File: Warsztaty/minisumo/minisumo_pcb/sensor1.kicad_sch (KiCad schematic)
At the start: 7 parts, among them U5 VL53L0CXV0DH1

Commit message: chyba gotowy schemat
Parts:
- C21, C22: footprint (none) -> Capacitor_SMD:C_0805_2012Metric_Pad1.18x1.45mm_HandSolder
- R10, R11, R12, R9: footprint (none) -> Resistor_SMD:R_0805_2012Metric_Pad1.20x1.40mm_HandSolder
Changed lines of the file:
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@@
 			)
 		)
-		(property "Footprint" ""
+		(property "Footprint" "Resistor_SMD:R_0805_2012Metric_Pad1.20x1.40mm_HandSolder"
 			(at 26.67 36.83 0)
 			(effects
@@
 			)
 		)
-		(property "Footprint" ""
+		(property "Footprint" "Resistor_SMD:R_0805_2012Metric_Pad1.20x1.40mm_HandSolder"
 			(at 38.1 36.83 0)
 			(effects
@@
 			)
 		)
-		(property "Footprint" ""
+		(property "Footprint" "Resistor_SMD:R_0805_2012Metric_Pad1.20x1.40mm_HandSolder"
 			(at 33.02 36.83 0)
 			(effects
@@
 			)
 		)
-		(property "Footprint" ""
+		(property "Footprint" "Capacitor_SMD:C_0805_2012Metric_Pad1.18x1.45mm_HandSolder"
 			(at 74.93 39.37 0)
 			(effects
@@
 			)
 		)
-		(property "Footprint" ""
+		(property "Footprint" "Resistor_SMD:R_0805_2012Metric_Pad1.20x1.40mm_HandSolder"
 			(at 43.18 36.83 0)
 			(effects
@@
 			)
 		)
-		(property "Footprint" ""
+		(property "Footprint" "Capacitor_SMD:C_0805_2012Metric_Pad1.18x1.45mm_HandSolder"
 			(at 69.85 39.37 0)
 			(effects

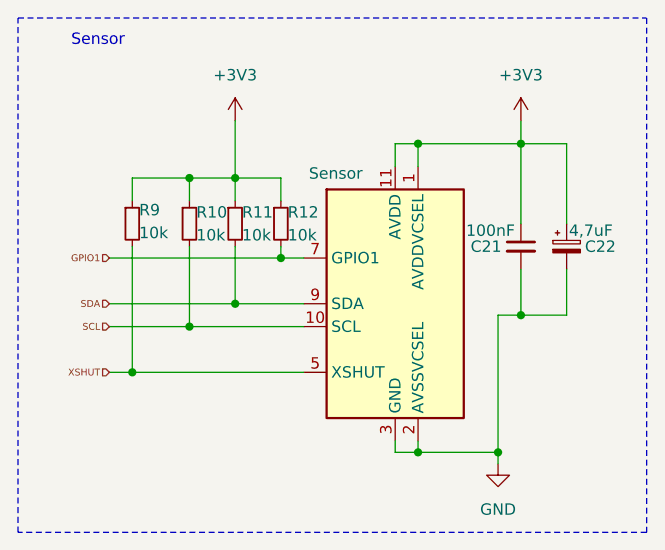
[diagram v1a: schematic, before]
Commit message: chyba gotowy schemat
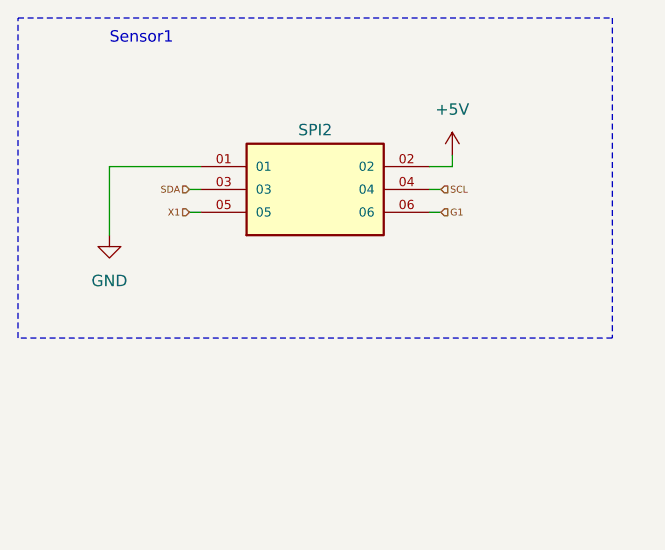
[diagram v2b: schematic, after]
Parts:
- removed C21: 100nF, Capacitor_SMD:C_0805_2012Metric_Pad1.18x1.45mm_HandSolder, symbol Device:C_Small
- removed C22: 4,7uF, Capacitor_SMD:C_0805_2012Metric_Pad1.18x1.45mm_HandSolder, symbol Device:C_Polarized_Small
- removed R10, R11, R12, R9: 10k, Resistor_SMD:R_0805_2012Metric_Pad1.20x1.40mm_HandSolder, symbol Device:R_Small
- removed U5: VL53L0CXV0DH1, Sensor_Distance:ST_VL53L1x, symbol Sensor_Distance:VL53L0CXV0DH1
- added SPI2: MTSW-103-23-F-D-230, MTSW-103-23-F-D-230:SAMTEC_MTSW-103-23-F-D-230, symbol MTSW-103-23-F-D-230:MTSW-103-23-F-D-230
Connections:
- net GND: now also SPI2.01
- net SCL: now also SPI2.04
- net SDA: now also SPI2.03
- new net +5V: SPI2.02
- new net G1: SPI2.06
- new net X1: SPI2.05
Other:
- note added: "Sensor1"
- note removed: "Sensor"
